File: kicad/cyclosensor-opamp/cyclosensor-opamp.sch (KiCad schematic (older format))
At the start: 11 parts, among them J1 RJ14, U1 LM358, U2 TCRT5000

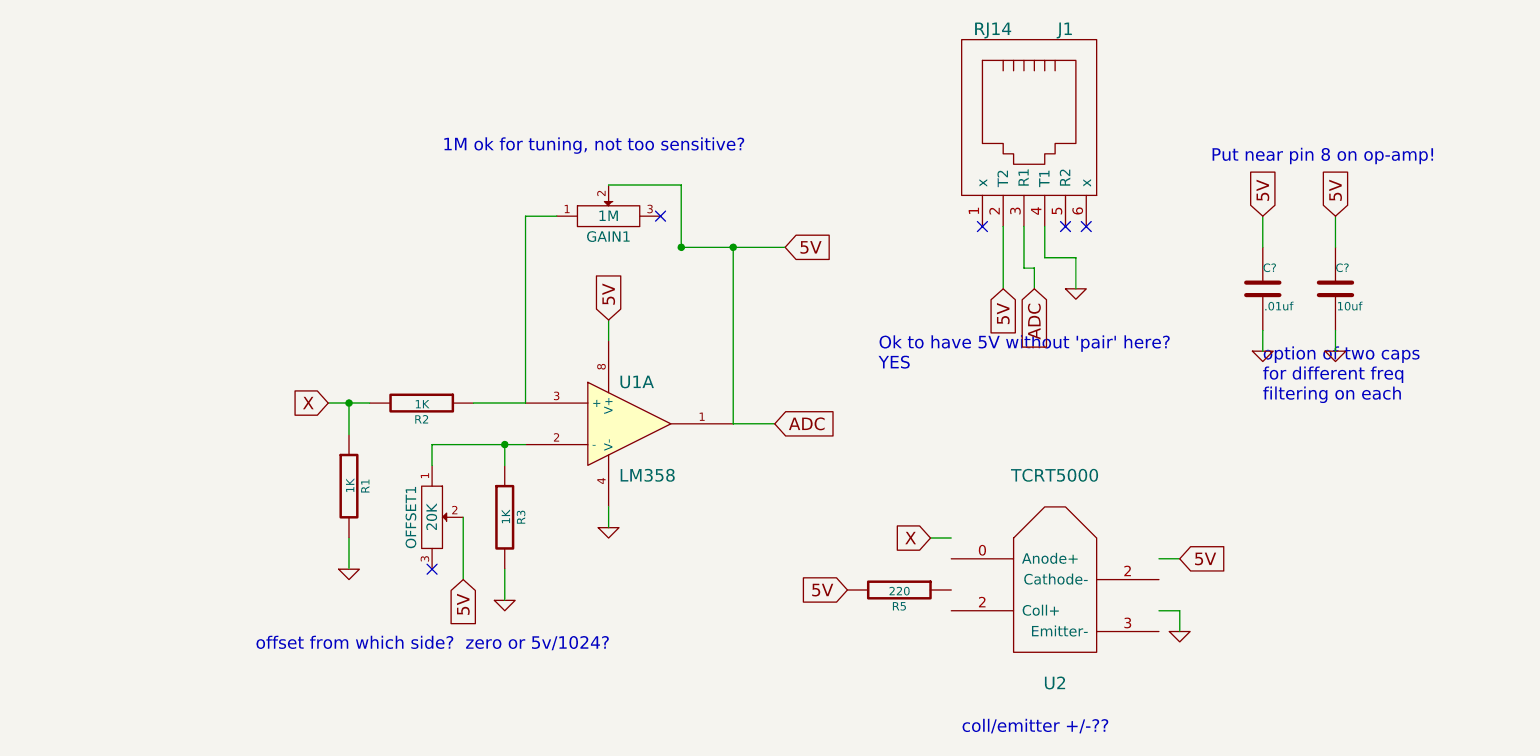
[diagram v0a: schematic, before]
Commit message: update tcrt5000
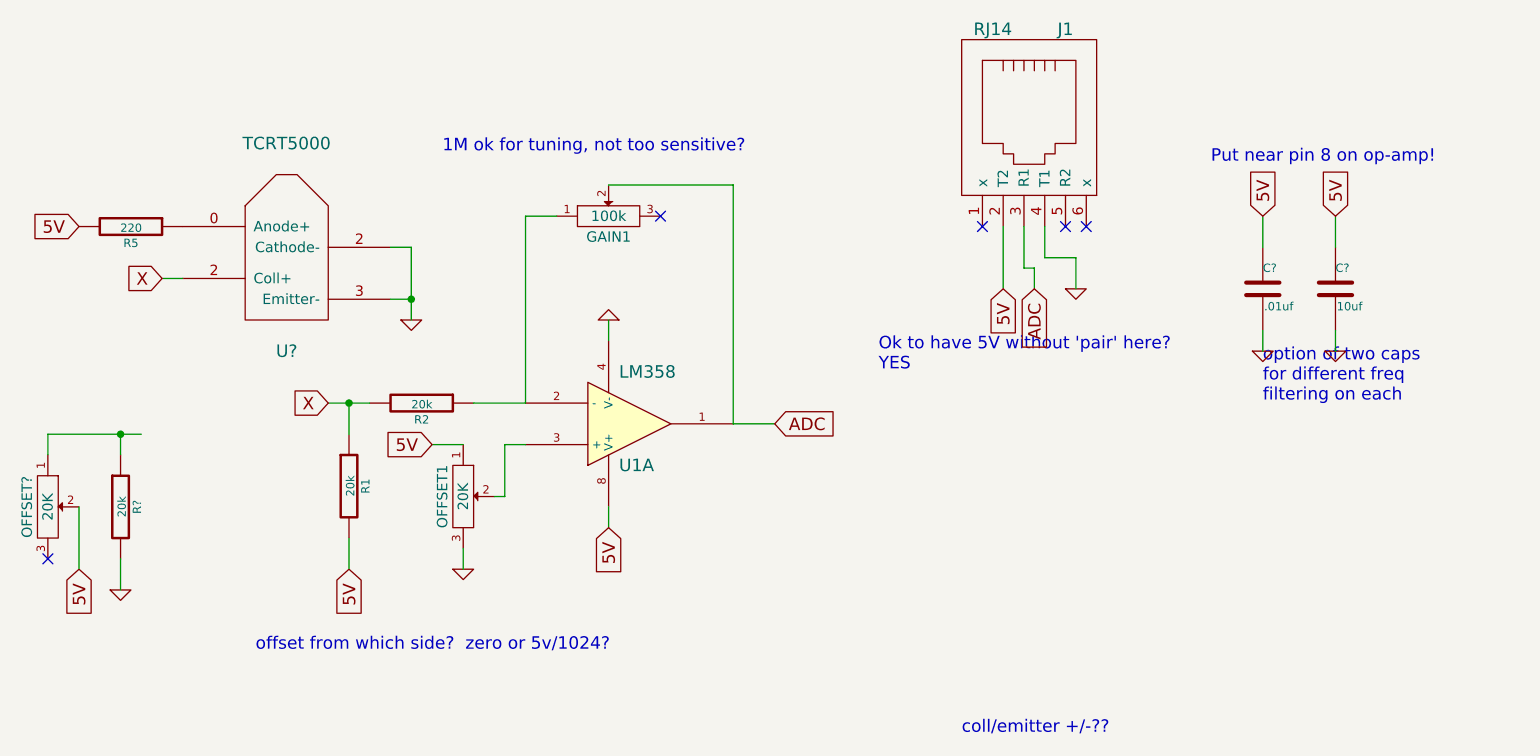
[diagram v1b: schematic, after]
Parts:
- removed R3: 1K, ~, symbol R
- removed U2: TCRT5000, ~, symbol TCRT5000
- added OFFSET?: 20K, ~, symbol POT
- added R?: 20k, ~, symbol R
- added U?: TCRT5000, ~, symbol TCRT5000
- GAIN1: value 1M -> 100k
- R1, R2: value 1K -> 20k
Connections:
- wire segments 33 -> 36
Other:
- moved on the sheet: OFFSET1, R5
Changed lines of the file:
@@
 Sheet 1 1
 Title ""
-Date "9 apr 2014"
+Date "12 apr 2014"
 Rev ""
 Comp ""
@@
 	1    0    0    -1
 $EndComp
-$Comp
-L TCRT5000 U2
-U 1 1 532FB873
-P 7050 5150
-F 0 "U2" H 7050 4600 60  0000 C CNN
-F 1 "TCRT5000" H 7050 5600 60  0000 C CNN
-F 2 "~" H 7050 5150 60  0000 C CNN
-F 3 "~" H 7050 5150 60  0000 C CNN
-	1    7050 5150
-	1    0    0    -1
-$EndComp
 Text GLabel 6800 3800 3    60   Input ~ 0
 5V
@@
 	1    0    0    -1
 $EndComp
-Text GLabel 4900 3950 1    60   Input ~ 0
+Text GLabel 4900 4950 3    60   Input ~ 0
 5V
 $Comp
 L GND #PWR02
 U 1 1 533B8353
-P 4900 4950
-F 0 "#PWR02" H 4900 4950 30  0001 C CNN
-F 1 "GND" H 4900 4880 30  0001 C CNN
-F 2 "" H 4900 4950 60  0000 C CNN
-F 3 "" H 4900 4950 60  0000 C CNN
-	1    4900 4950
-	1    0    0    -1
+P 4900 3950
+F 0 "#PWR02" H 4900 3950 30  0001 C CNN
+F 1 "GND" H 4900 3880 30  0001 C CNN
+F 2 "" H 4900 3950 60  0000 C CNN
+F 3 "" H 4900 3950 60  0000 C CNN
+	1    4900 3950
+	-1   0    0    1
 $EndComp
 $Comp
@@
 F 3 "" H 5000 4450 60  0000 C CNN
 	1    5000 4450
-	1    0    0    -1
+	1    0    0    1
 $EndComp
 $Comp
@@
 P 4000 4350
 F 0 "R2" V 4080 4350 40  0000 C CNN
-F 1 "1K" V 4007 4351 40  0000 C CNN
+F 1 "20k" V 4007 4351 40  0000 C CNN
 F 2 "~" V 3930 4350 30  0000 C CNN
 F 3 "~" H 4000 4350 30  0000 C CNN
@@
 ADC
 $Comp
-L R R3
-U 1 1 533B9B66
-P 4400 4900
-F 0 "R3" V 4480 4900 40  0000 C CNN
-F 1 "1K" V 4407 4901 40  0000 C CNN
-F 2 "~" V 4330 4900 30  0000 C CNN
-F 3 "~" H 4400 4900 30  0000 C CNN
-	1    4400 4900
-	1    0    0    -1
-$EndComp
-$Comp
 L R R1
 U 1 1 533B9B87
 P 3650 4750
 F 0 "R1" V 3730 4750 40  0000 C CNN
-F 1 "1K" V 3657 4751 40  0000 C CNN
+F 1 "20k" V 3657 4751 40  0000 C CNN
 F 2 "~" V 3580 4750 30  0000 C CNN
 F 3 "~" H 3650 4750 30  0000 C CNN
@@
 	1    0    0    -1
 $EndComp
-Text GLabel 5750 3600 2    60   Input ~ 0
-5V
-Text GLabel 7650 5100 2    60   Input ~ 0
-5V
-$Comp
-L GND #PWR03
-U 1 1 533B9C11
-P 3650 5150
-F 0 "#PWR03" H 3650 5150 30  0001 C CNN
-F 1 "GND" H 3650 5080 30  0001 C CNN
-F 2 "" H 3650 5150 60  0000 C CNN
-F 3 "" H 3650 5150 60  0000 C CNN
-	1    3650 5150
-	1    0    0    -1
-$EndComp
-$Comp
-L GND #PWR04
-U 1 1 533B9C20
-P 4400 5300
-F 0 "#PWR04" H 4400 5300 30  0001 C CNN
-F 1 "GND" H 4400 5230 30  0001 C CNN
-F 2 "" H 4400 5300 60  0000 C CNN
-F 3 "" H 4400 5300 60  0000 C CNN
-	1    4400 5300
-	1    0    0    -1
-$EndComp
-Text GLabel 6450 5000 0    60   Input ~ 0
+Text GLabel 2750 3750 0    60   Input ~ 0
 X
 Text GLabel 3550 4350 0    60   Input ~ 0
 X
-Text GLabel 6050 5250 0    60   Input ~ 0
+Text GLabel 2350 3500 0    60   Input ~ 0
 5V
 $Comp
 L GND #PWR05
 U 1 1 533B9F2F
-P 7650 5450
-F 0 "#PWR05" H 7650 5450 30  0001 C CNN
-F 1 "GND" H 7650 5380 30  0001 C CNN
-F 2 "" H 7650 5450 60  0000 C CNN
-F 3 "" H 7650 5450 60  0000 C CNN
-	1    7650 5450
+P 3950 3950
+F 0 "#PWR05" H 3950 3950 30  0001 C CNN
+F 1 "GND" H 3950 3880 30  0001 C CNN
+F 2 "" H 3950 3950 60  0000 C CNN
+F 3 "" H 3950 3950 60  0000 C CNN
+	1    3950 3950
 	1    0    0    -1
 $EndComp
@@
 L R R5
 U 1 1 533B9FB6
-P 6300 5250
-F 0 "R5" V 6380 5250 40  0000 C CNN
-F 1 "220" V 6307 5251 40  0000 C CNN
-F 2 "~" V 6230 5250 30  0000 C CNN
-F 3 "~" H 6300 5250 30  0000 C CNN
-	1    6300 5250
+P 2600 3500
+F 0 "R5" V 2680 3500 40  0000 C CNN
+F 1 "220" V 2607 3501 40  0000 C CNN
+F 2 "~" V 2530 3500 30  0000 C CNN
+F 3 "~" H 2600 3500 30  0000 C CNN
+	1    2600 3500
 	0    1    1    0
 $EndComp
 NoConn ~ 6700 3500
 NoConn ~ 7200 3500
-Wire Wire Line
-	7000 3500 7000 3650
-Wire Wire Line
-	7000 3650 7150 3650
-Wire Wire Line
-	4500 3450 4500 4350
-Wire Wire Line
-	4500 4350 4250 4350
-Wire Wire Line
-	3550 4350 3750 4350
-Wire Wire Line
-	3650 4350 3650 4500
-Connection ~ 3650 4350
-Wire Wire Line
-	6450 5000 6550 5000
-Wire Wire Line
-	7650 5100 7550 5100
-Wire Wire Line
-	5500 4450 5700 4450
-Wire Wire Line
-	4050 4550 4500 4550
-Wire Wire Line
-	4400 4550 4400 4650
-Wire Wire Line
-	4400 5150 4400 5300
-Wire Wire Line
-	3650 5000 3650 5150
-Wire Wire Line
-	5500 4450 5500 3600
-Connection ~ 5500 3600
-Wire Wire Line
-	4900 3950 4900 4050
-Wire Wire Line
-	6900 3500 6900 3700
-Wire Wire Line
-	6900 3700 6950 3700
-Wire Wire Line
-	6950 3700 6950 3800
-Wire Wire Line
-	7550 5350 7650 5350
-Wire Wire Line
-	7650 5350 7650 5450
 $Comp
 L POT GAIN1
@@
 P 4900 3450
 F 0 "GAIN1" H 4900 3350 50  0000 C CNN
-F 1 "1M" H 4900 3450 50  0000 C CNN
+F 1 "100k" H 4900 3450 50  0000 C CNN
 F 2 "~" H 4900 3450 60  0000 C CNN
 F 3 "~" H 4900 3450 60  0000 C CNN
@@
 	1    0    0    -1
 $EndComp
-Wire Wire Line
-	4500 3450 4650 3450
-Wire Wire Line
-	4900 3300 5250 3300
-Wire Wire Line
-	5250 3300 5250 3600
-Connection ~ 5250 3600
 NoConn ~ 5150 3450
-Wire Wire Line
-	5250 3600 5750 3600
 $Comp
 L POT OFFSET1
 U 1 1 533BA12C
-P 4050 4900
-F 0 "OFFSET1" H 4050 4800 50  0000 C CNN
-F 1 "20K" H 4050 4900 50  0000 C CNN
-F 2 "~" H 4050 4900 60  0000 C CNN
-F 3 "~" H 4050 4900 60  0000 C CNN
-	1    4050 4900
+P 4200 4800
+F 0 "OFFSET1" H 4200 4700 50  0000 C CNN
+F 1 "20K" H 4200 4800 50  0000 C CNN
+F 2 "~" H 4200 4800 60  0000 C CNN
+F 3 "~" H 4200 4800 60  0000 C CNN
+	1    4200 4800
 	0    1    1    0
 $EndComp
-Wire Wire Line
-	4050 4550 4050 4650
-Connection ~ 4400 4550
-Text GLabel 4200 5200 3    60   Input ~ 0
-5V
-Wire Wire Line
-	4200 4900 4200 5200
-NoConn ~ 4050 5150
-Wire Wire Line
-	4900 4850 4900 4950
-Wire Wire Line
-	7150 3650 7150 3800
+Text GLabel 4050 4550 0    60   Input ~ 0
+5V
 NoConn ~ 7100 3500
-Wire Wire Line
-	6800 3800 6800 3500
 Text Notes 6200 4200 0    60   ~ 0
 Ok to have 5V without 'pair' here?  \nYES
@@
 	1    0    0    -1
 $EndComp
-Wire Wire Line
-	8050 4000 8050 4100
-Wire Wire Line
-	8050 3450 8050 3600
 Text Notes 7800 3200 0    60   ~ 0
 Put near pin 8 on op-amp!
@@
 	1    0    0    -1
 $EndComp
-Wire Wire Line
-	8400 4000 8400 4100
-Wire Wire Line
-	8400 3450 8400 3600
 Text Notes 8050 4350 0    60   ~ 0
 option of two caps \nfor different freq\nfiltering on each
+$Comp
+L TCRT5000 U?
+U 1 1 53499E1E
+P 3350 3550
+F 0 "U?" H 3350 3000 60  0000 C CNN
+F 1 "TCRT5000" H 3350 4000 60  0000 C CNN
+F 2 "~" H 3350 3550 60  0000 C CNN
+F 3 "~" H 3350 3550 60  0000 C CNN
+	1    3350 3550
+	1    0    0    -1
+$EndComp
+Wire Wire Line
+	7000 3500 7000 3650
+Wire Wire Line
+	7000 3650 7150 3650
+Wire Wire Line
+	4500 3450 4500 4350
+Wire Wire Line
+	4500 4350 4250 4350
+Wire Wire Line
+	3550 4350 3750 4350
+Wire Wire Line
+	3650 4350 3650 4500
+Connection ~ 3650 4350
+Wire Wire Line
+	2750 3750 2850 3750
+Wire Wire Line
+	5500 4450 5700 4450
+Wire Wire Line
+	3650 5000 3650 5150
+Wire Wire Line
+	4900 3950 4900 4050
+Wire Wire Line
+	6900 3500 6900 3700
+Wire Wire Line
+	6900 3700 6950 3700
+Wire Wire Line
+	6950 3700 6950 3800
+Wire Wire Line
+	3850 3850 3950 3850
+Wire Wire Line
+	3950 3600 3950 3950
+Wire Wire Line
+	4500 3450 4650 3450
+Wire Wire Line
+	4900 4850 4900 4950
+Wire Wire Line
+	7150 3650 7150 3800
+Wire Wire Line
+	6800 3800 6800 3500
+Wire Wire Line
+	8050 4000 8050 4100
+Wire Wire Line
+	8050 3450 8050 3600
+Wire Wire Line
+	8400 4000 8400 4100
+Wire Wire Line
+	8400 3450 8400 3600
+Wire Wire Line
+	4900 3300 5500 3300
+Wire Wire Line
+	5500 3300 5500 4450
+Wire Wire Line
+	3950 3600 3850 3600
+Connection ~ 3950 3850
+Text GLabel 3650 5150 3    60   Input ~ 0
+5V
+$Comp
+L R R?
+U 1 1 5349C83F
+P 2550 4850
+F 0 "R?" V 2630 4850 40  0000 C CNN
+F 1 "20k" V 2557 4851 40  0000 C CNN
+F 2 "~" V 2480 4850 30  0000 C CNN
+F 3 "~" H 2550 4850 30  0000 C CNN
+	1    2550 4850
+	1    0    0    -1
+$EndComp
+$Comp
+L GND #PWR?
+U 1 1 5349C845
+P 2550 5250
+F 0 "#PWR?" H 2550 5250 30  0001 C CNN
+F 1 "GND" H 2550 5180 30  0001 C CNN
+F 2 "" H 2550 5250 60  0000 C CNN
+F 3 "" H 2550 5250 60  0000 C CNN
+	1    2550 5250
+	1    0    0    -1
+$EndComp
+$Comp
+L POT OFFSET?
+U 1 1 5349C84B
+P 2200 4850
+F 0 "OFFSET?" H 2200 4750 50  0000 C CNN
+F 1 "20K" H 2200 4850 50  0000 C CNN
+F 2 "~" H 2200 4850 60  0000 C CNN
+F 3 "~" H 2200 4850 60  0000 C CNN
+	1    2200 4850
+	0    1    1    0
+$EndComp
+Text GLabel 2350 5150 3    60   Input ~ 0
+5V
+NoConn ~ 2200 5100
+Wire Wire Line
+	2200 4500 2650 4500
+Wire Wire Line
+	2550 4500 2550 4600
+Wire Wire Line
+	2550 5100 2550 5250
+Wire Wire Line
+	2200 4500 2200 4600
+Connection ~ 2550 4500
+Wire Wire Line
+	2350 4850 2350 5150
+$Comp
+L GND #PWR?
+U 1 1 5349C88D
+P 4200 5150
+F 0 "#PWR?" H 4200 5150 30  0001 C CNN
+F 1 "GND" H 4200 5080 30  0001 C CNN
+F 2 "" H 4200 5150 60  0000 C CNN
+F 3 "" H 4200 5150 60  0000 C CNN
+	1    4200 5150
+	1    0    0    -1
+$EndComp
+Wire Wire Line
+	4350 4800 4400 4800
+Wire Wire Line
+	4400 4800 4400 4550
+Wire Wire Line
+	4400 4550 4500 4550
+Wire Wire Line
+	4050 4550 4200 4550
+Wire Wire Line
+	4200 5150 4200 5050
 $EndSCHEMATC
